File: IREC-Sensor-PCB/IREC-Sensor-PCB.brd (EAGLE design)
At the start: 66 x 55.9 mm, 9 parts, among them K1 RELAY-SPDT-JQX-15F

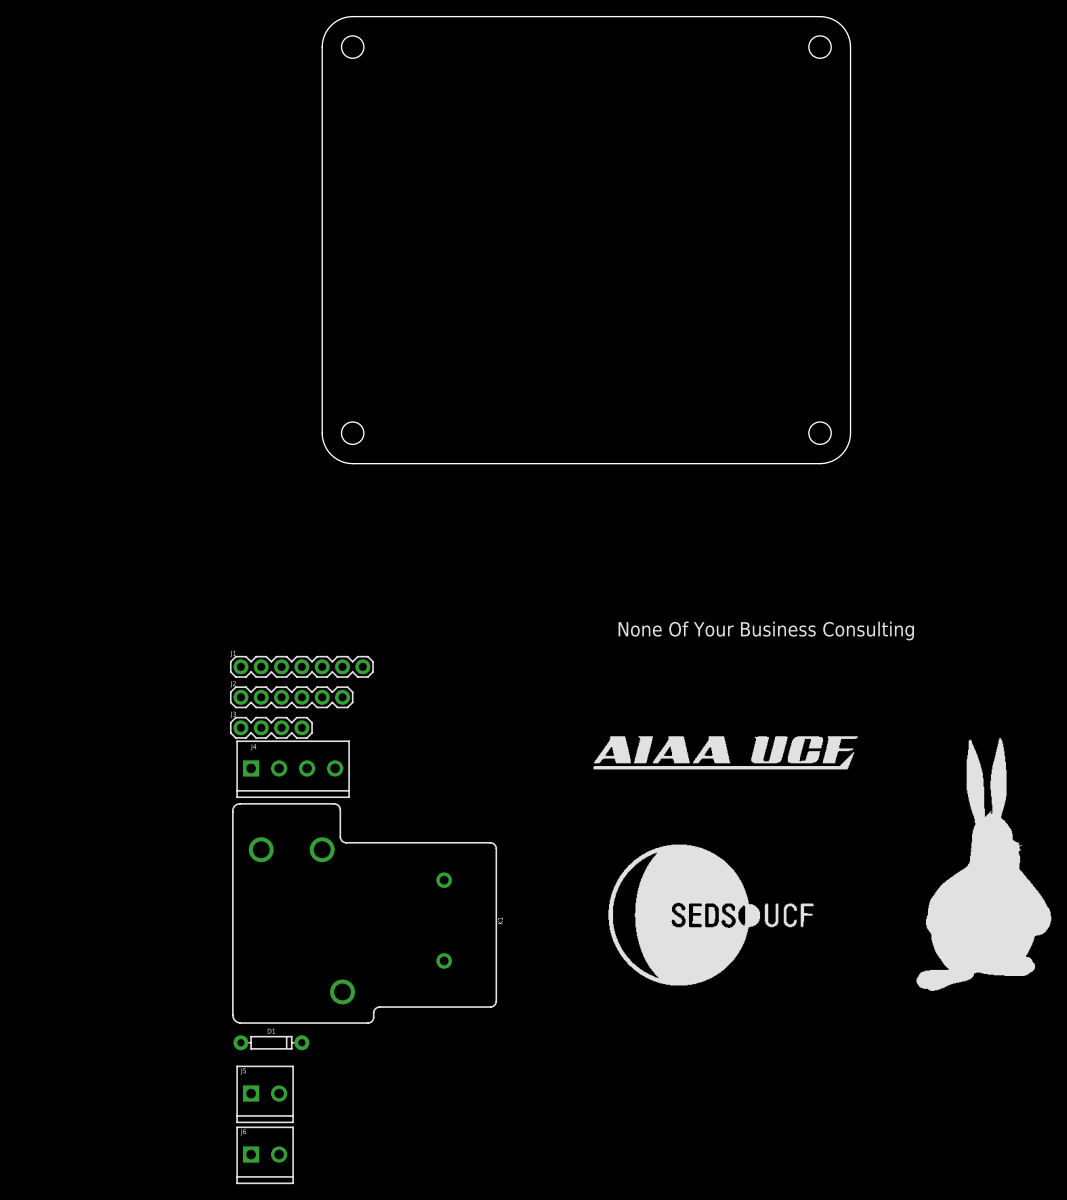
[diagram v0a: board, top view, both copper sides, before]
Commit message: Completed layout
Completed board layout
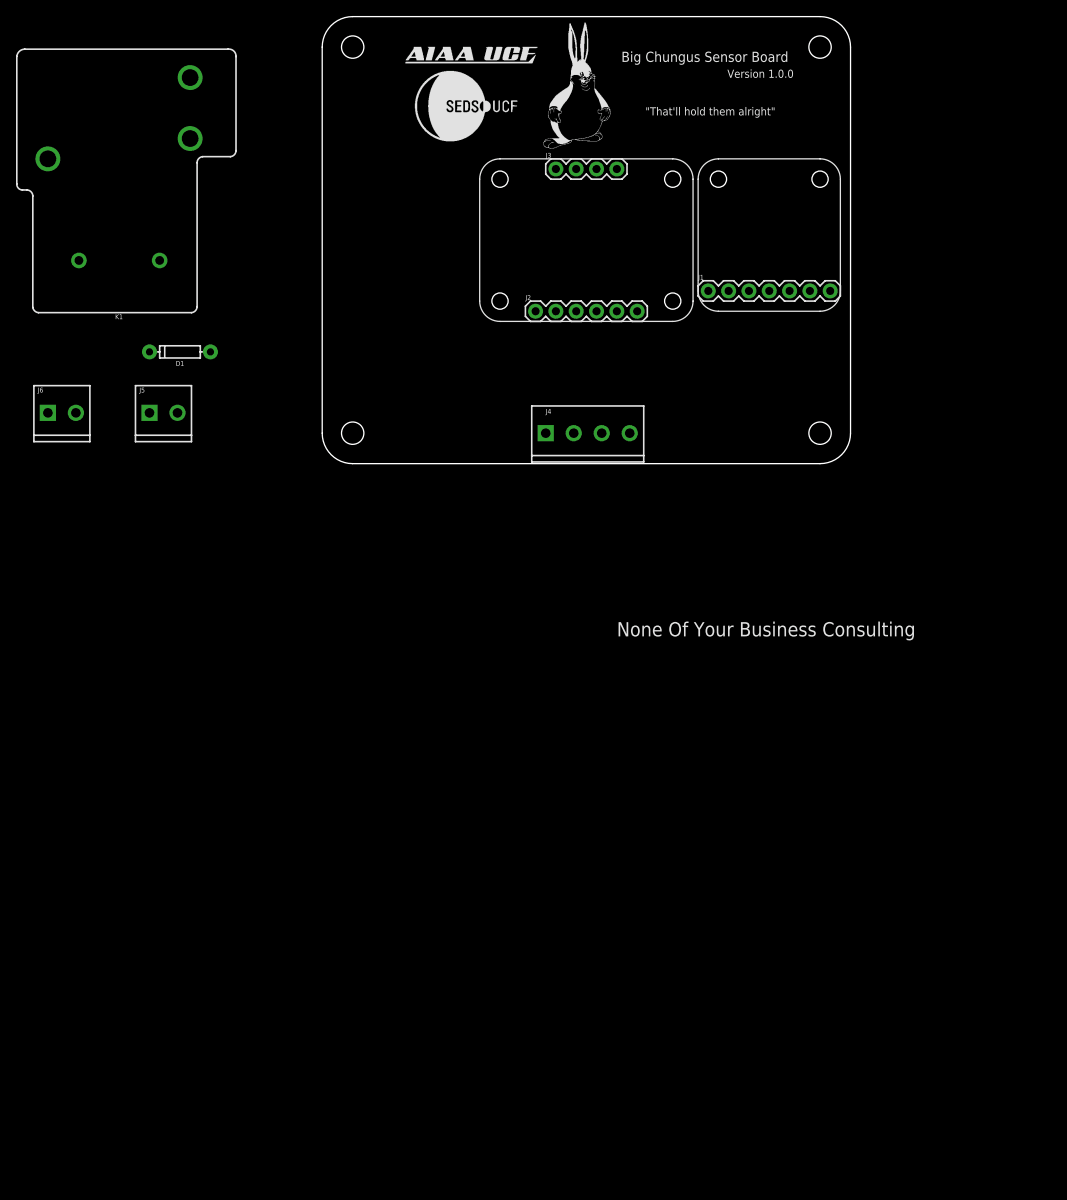
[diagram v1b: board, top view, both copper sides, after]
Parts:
- moved J6 96.1 mm to (-34.3, 6.35)
- moved D1 87.1 mm to (-17.8, 14.0), turned to 180 degrees
- moved J5 86.0 mm to (-21.6, 6.35)
- moved K1 80.2 mm to (-16.5, 25.4), turned to 270 degrees
- moved J3 80.2 mm to (29.2, 36.8)
- moved J1 75.0 mm to (48.3, 21.6)
- moved J2 60.7 mm to (26.7, 19.1)
- moved J4 55.8 mm to (27.9, 3.81)
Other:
- board text added: ""That'll hold them alright""
- board text added: "Big Chungus Sensor Board"
- board text added: "Version 1.0.0"
